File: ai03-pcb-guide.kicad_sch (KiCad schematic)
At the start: 24 parts, among them SW1 SW_Push, U2 ATmega32U4-A, Y1 16Mhz

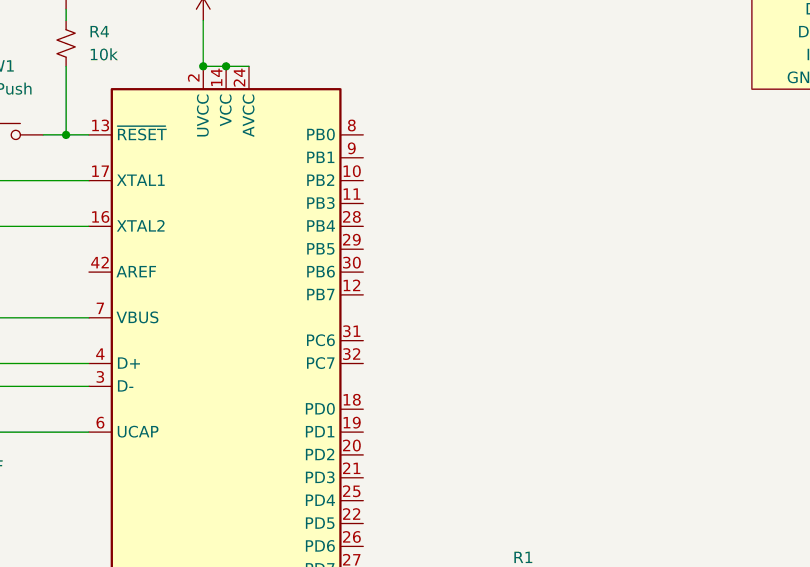
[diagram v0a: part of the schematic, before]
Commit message: Done routing
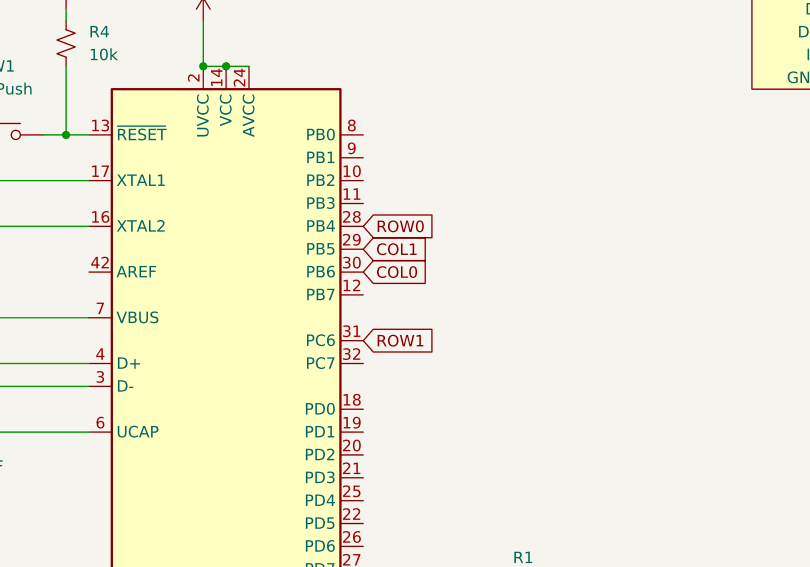
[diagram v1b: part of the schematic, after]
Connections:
- net COL0: now also U2.30 (PB6)
- net COL1: now also U2.29 (PB5)
- net ROW0: now also U2.28 (PB4)
- net ROW1: now also U2.31 (PC6)
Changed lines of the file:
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@@
+    )
+  )
+  (global_label "ROW0" (shape input) (at 134.62 81.28 0) (fields_autoplaced)
+    (effects (font (size 1.27 1.27)) (justify left))
+    (property "Intersheetrefs" "${INTERSHEET_REFS}" (at 142.7872 81.28 0)
+      (effects (font (size 1.27 1.27)) (justify left) hide)
     )
   )
@@
     )
   )
+  (global_label "COL0" (shape input) (at 134.62 86.36 0) (fields_autoplaced)
+    (effects (font (size 1.27 1.27)) (justify left))
+    (property "Intersheetrefs" "${INTERSHEET_REFS}" (at 142.3639 86.36 0)
+      (effects (font (size 1.27 1.27)) (justify left) hide)
+    )
+  )
   (global_label "COL0" (shape input) (at 217.17 101.6 90) (fields_autoplaced)
     (effects (font (size 1.27 1.27)) (justify left))
@@
     )
   )
+  (global_label "COL1" (shape input) (at 134.62 83.82 0) (fields_autoplaced)
+    (effects (font (size 1.27 1.27)) (justify left))
+    (property "Intersheetrefs" "${INTERSHEET_REFS}" (at 142.3639 83.82 0)
+      (effects (font (size 1.27 1.27)) (justify left) hide)
+    )
+  )
   (global_label "D-" (shape input) (at 68.58 99.06 180) (fields_autoplaced)
     (effects (font (size 1.27 1.27)) (justify right))
@@
     )
   )
+  (global_label "ROW1" (shape input) (at 134.62 93.98 0) (fields_autoplaced)
+    (effects (font (size 1.27 1.27)) (justify left))
+    (property "Intersheetrefs" "${INTERSHEET_REFS}" (at 142.7872 93.98 0)
+      (effects (font (size 1.27 1.27)) (justify left) hide)
+    )
+  )
